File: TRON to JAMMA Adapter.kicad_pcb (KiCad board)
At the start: 2 copper layers, 111 x 98.7 mm, 58 parts, among them P1 1K, P2 10K, P3 1K, U1 74LS86, U2A 74LS191, U2B 74LS191, U3 NE555, U4 LM386, U5 NE555

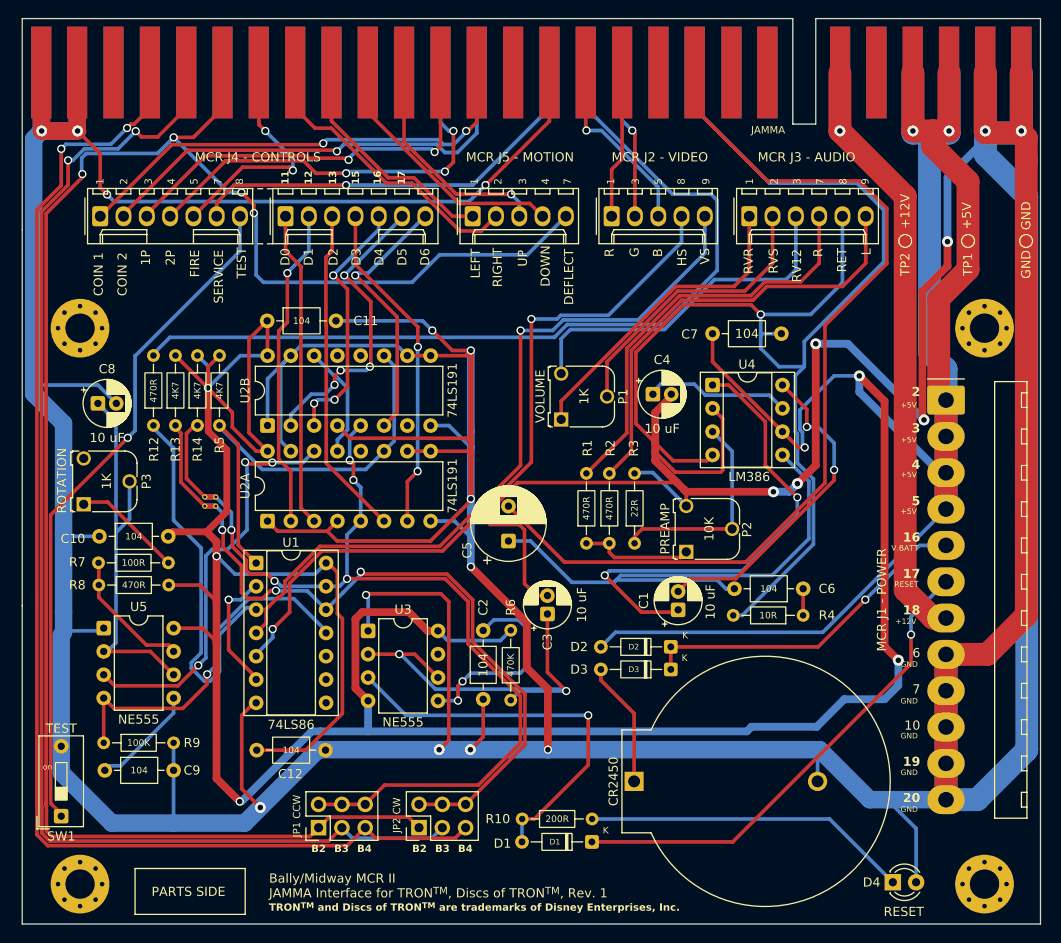
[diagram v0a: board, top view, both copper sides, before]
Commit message: slightly widen
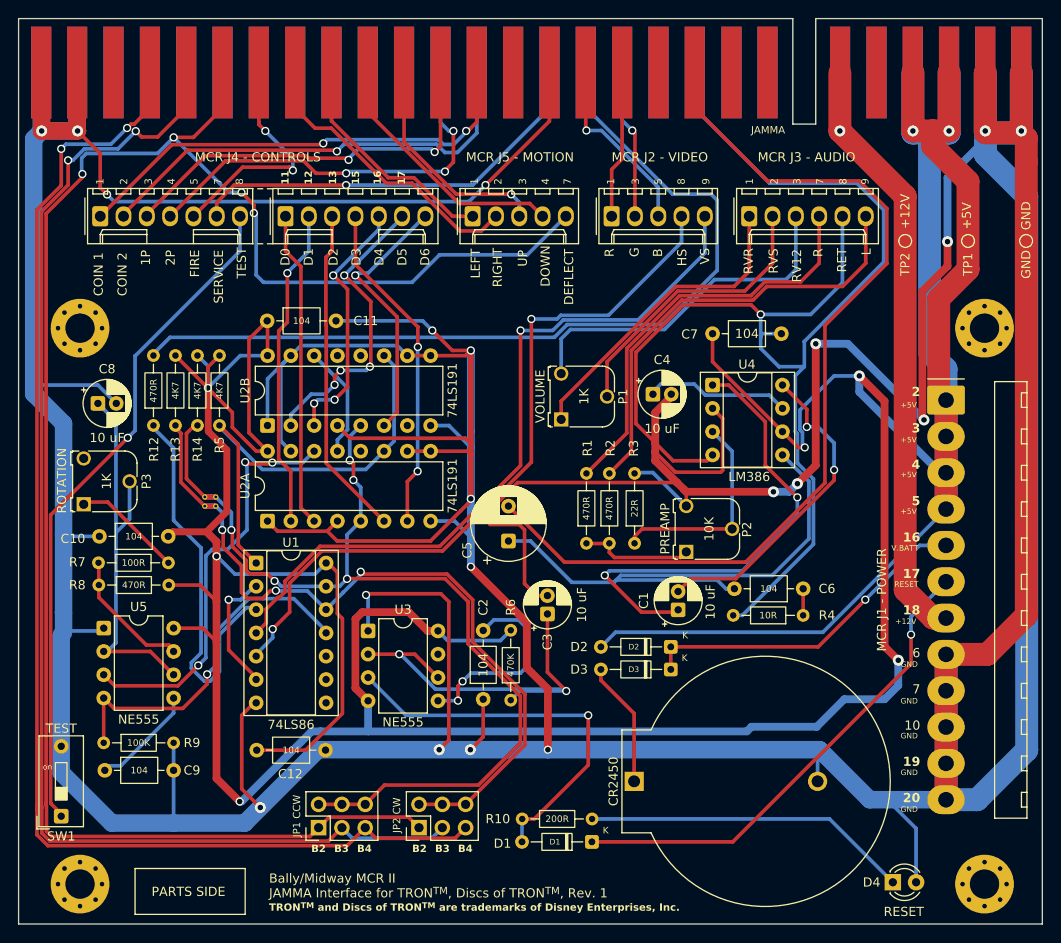
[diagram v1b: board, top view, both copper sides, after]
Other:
- board size 111 x 98.7 mm -> 111.6 x 98.7 mm
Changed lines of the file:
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@@
 	(gr_poly
 		(pts
-			(xy 173.5 56.550005) (xy 176 56.550005) (xy 176 45.05) (xy 200.500004 45.05) (xy 200.500004 68.050005)
-			(xy 200.5 68.050005) (xy 200.5 109.050005) (xy 200.5 143.75) (xy 89.5 143.75) (xy 89.5 109.050005)
-			(xy 89.499997 109.050005) (xy 89.499997 68.050005) (xy 89.499997 45.05) (xy 173.5 45.05)
+			(xy 173.5 56.550005) (xy 176 56.550005) (xy 176 45.05) (xy 200.700004 45.05) (xy 200.7 143.75) (xy 89.1 143.75)
+			(xy 89.099997 45.05) (xy 173.5 45.05)
 		)
 		(stroke
